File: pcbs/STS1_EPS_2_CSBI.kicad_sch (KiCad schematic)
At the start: 10 parts

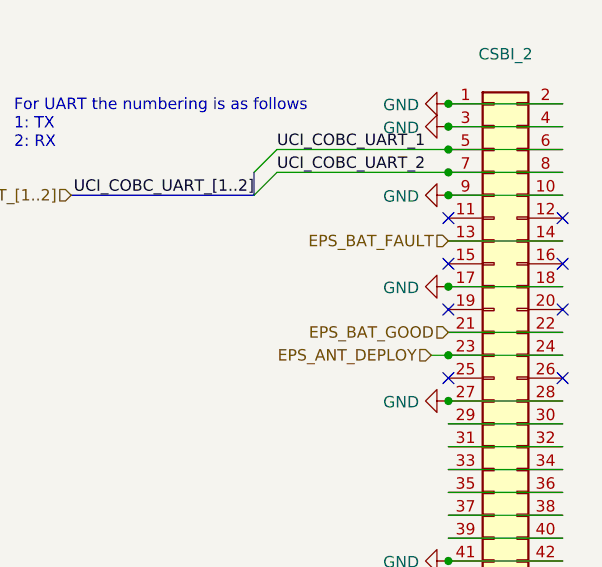
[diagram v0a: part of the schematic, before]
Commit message: Intermediate commit.
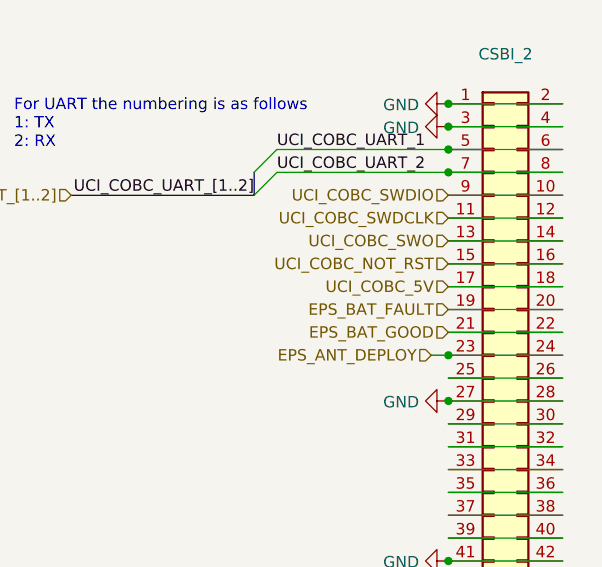
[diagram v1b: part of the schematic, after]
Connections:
- net EPS_BAT_FAULT: now also CSBI_2.19 (Pin_19), CSBI_2.20 (Pin_20); no longer CSBI_2.13 (Pin_13), CSBI_2.14 (Pin_14)
- net GND: no longer CSBI_2.10 (Pin_10), CSBI_2.17 (Pin_17), CSBI_2.18 (Pin_18), CSBI_2.9 (Pin_9)
- net UCI_COBC_SWDCLK: now reaches CSBI_2.11 (Pin_11)
- net UCI_COBC_SWDCLK: now also CSBI_2.12 (Pin_12)
- net UCI_COBC_NOT_RST: now reaches CSBI_2.15 (Pin_15)
- net UCI_COBC_NOT_RST: now also CSBI_2.16 (Pin_16)
- net at CSBI_2.25 (Pin_25): now also CSBI_2.26 (Pin_26)
- new net UCI_COBC_5V: CSBI_2.17 (Pin_17), CSBI_2.18 (Pin_18)
- new net UCI_COBC_SWDIO: CSBI_2.10 (Pin_10), CSBI_2.9 (Pin_9)
- new net UCI_COBC_SWO: CSBI_2.13 (Pin_13), CSBI_2.14 (Pin_14)
- no-connect marks 8 -> 0
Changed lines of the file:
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@@
-	)
-	(junction
-		(at 193.04 63.5)
-		(diameter 0)
-		(color 0 0 0 0)
 	)
 	(junction
@@
 	)
 	(junction
-		(at 193.04 53.34)
-		(diameter 0)
-		(color 0 0 0 0)
-	)
-	(junction
 		(at 87.63 44.45)
 		(diameter 0)
@@
 		(color 0 0 0 0)
 	)
-	(no_connect
-		(at 193.04 73.66)
-	)
-	(no_connect
-		(at 205.74 55.88)
-	)
-	(no_connect
-		(at 193.04 55.88)
-	)
-	(no_connect
-		(at 205.74 66.04)
-	)
-	(no_connect
-		(at 193.04 60.96)
-	)
-	(no_connect
-		(at 193.04 66.04)
-	)
-	(no_connect
-		(at 205.74 60.96)
-	)
-	(no_connect
-		(at 205.74 73.66)
-	)
 	(bus_entry
 		(at 171.45 50.8)
@@
 	(wire
 		(pts
+			(xy 193.04 55.88) (xy 205.74 55.88)
+		)
+		(stroke
+			(width 0)
+			(type default)
+		)
+	)
+	(wire
+		(pts
 			(xy 80.01 49.53) (xy 87.63 49.53)
 		)
@@
 	(wire
 		(pts
+			(xy 193.04 60.96) (xy 205.74 60.96)
+		)
+		(stroke
+			(width 0)
+			(type default)
+		)
+	)
+	(wire
+		(pts
 			(xy 193.04 81.28) (xy 205.74 81.28)
 		)
@@
 	(wire
 		(pts
+			(xy 193.04 73.66) (xy 205.74 73.66)
+		)
+		(stroke
+			(width 0)
+			(type default)
+		)
+	)
+	(wire
+		(pts
 			(xy 193.04 48.26) (xy 205.74 48.26)
 		)
@@
 		(pts
 			(xy 173.99 48.26) (xy 193.04 48.26)
+		)
+		(stroke
+			(width 0)
+			(type default)
+		)
+	)
+	(wire
+		(pts
+			(xy 193.04 66.04) (xy 205.74 66.04)
 		)
 		(stroke
@@
 			)
 			(justify right bottom)
+		)
+	)
+	(hierarchical_label "UCI_COBC_SWO"
+		(shape input)
+		(at 193.04 58.42 180)
+		(fields_autoplaced yes)
+		(effects
+			(font
+				(size 1.27 1.27)
+			)
+			(justify right)
 		)
 	)
@@
 		)
 	)
+	(hierarchical_label "UCI_COBC_NOT_RST"
+		(shape input)
+		(at 193.04 60.96 180)
+		(fields_autoplaced yes)
+		(effects
+			(font
+				(size 1.27 1.27)
+			)
+			(justify right)
+		)
+	)
 	(hierarchical_label "VOUT"
 		(shape input)
@@
 		)
 	)
+	(hierarchical_label "UCI_COBC_5V"
+		(shape input)
+		(at 193.04 63.5 180)
+		(fields_autoplaced yes)
+		(effects
+			(font
+				(size 1.27 1.27)
+			)
+			(justify right)
+		)
+	)
 	(hierarchical_label "VOUT"
 		(shape input)
@@
 		)
 	)
+	(hierarchical_label "UCI_COBC_SWDCLK"
+		(shape input)
+		(at 193.04 55.88 180)
+		(fields_autoplaced yes)
+		(effects
+			(font
+				(size 1.27 1.27)
+			)
+			(justify right)
+		)
+	)
 	(hierarchical_label "EPS_BAT_GOOD"
 		(shape input)
@@
 		)
 	)
+	(hierarchical_label "UCI_COBC_SWDIO"
+		(shape input)
+		(at 193.04 53.34 180)
+		(fields_autoplaced yes)
+		(effects
+			(font
+				(size 1.27 1.27)
+			)
+			(justify right)
+		)
+	)
 	(hierarchical_label "EPS_BAT_FAULT"
 		(shape input)
-		(at 193.04 58.42 180)
+		(at 193.04 66.04 180)
 		(fields_autoplaced yes)
 		(effects
@@
 	(symbol
 		(lib_id "power:GND")
-		(at 193.04 63.5 270)
-		(unit 1)
-		(exclude_from_sim no)
-		(in_bom yes)
-		(on_board yes)
-		(dnp no)
-		(property "Reference" "#PWR017"
-			(at 186.69 63.5 0)
-			(effects
-				(font
-					(size 1.27 1.27)
-				)
-				(hide yes)
-			)
-		)
-		(property "Value" "GND"
-			(at 189.7888 63.627 90)
-			(effects
-				(font
-					(size 1.27 1.27)
-				)
-				(justify right)
-			)
-		)
-		(property "Footprint" ""
-			(at 193.04 63.5 0)
-			(effects
-				(font
-					(size 1.27 1.27)
-				)
-				(hide yes)
-			)
-		)
-		(property "Datasheet" ""
-			(at 193.04 63.5 0)
-			(effects
-				(font
-					(size 1.27 1.27)
-				)
-				(hide yes)
-			)
-		)
-		(property "Description" ""
-			(at 193.04 63.5 0)
-			(effects
-				(font
-					(size 1.27 1.27)
-				)
-				(hide yes)
-			)
-		)
-		(pin "1"
-		)
-		(instances
-			(project "STS1_EPS_2"
-				(path "/38c03ff7-ea47-4d00-b37d-ddcaa7d87722/565e35d1-cb7b-4a86-8e2f-32bed42f487e"
-					(reference "#PWR017")
-					(unit 1)
-				)
-			)
-		)
-	)
-	(symbol
-		(lib_id "power:GND")
 		(at 193.04 93.98 270)
 		(unit 1)
@@
 					(unit 1)
 				)
-			)
-		)
-	)
-	(symbol
-		(lib_id "power:GND")
-		(at 193.04 53.34 270)
-		(unit 1)
-		(exclude_from_sim no)
-		(in_bom yes)
-		(on_board yes)
-		(dnp no)
-		(property "Reference" "#PWR016"
-			(at 186.69 53.34 0)
-			(effects
-				(font
-					(size 1.27 1.27)
-				)
-				(hide yes)
-			)
-		)
-		(property "Value" "GND"
-			(at 189.7888 53.467 90)
-			(effects
-				(font
-					(size 1.27 1.27)
-				)
-				(justify right)
-			)
-		)
-		(property "Footprint" ""
-			(at 193.04 53.34 0)
-			(effects
-				(font
-					(size 1.27 1.27)
-				)
-				(hide yes)
-			)
-		)
-		(property "Datasheet" ""
-			(at 193.04 53.34 0)
-			(effects
-				(font
-					(size 1.27 1.27)
-				)
-				(hide yes)
-			)
-		)
-		(property "Description" ""
-			(at 193.04 53.34 0)
-			(effects
-				(font
-					(size 1.27 1.27)
-				)
-				(hide yes)
-			)
-		)
-		(pin "1"
-		)
-		(instances
-			(project "STS1_EPS_2"
-				(path "/38c03ff7-ea47-4d00-b37d-ddcaa7d87722/565e35d1-cb7b-4a86-8e2f-32bed42f487e"
-					(reference "#PWR016")
-					(unit 1)
-				)
